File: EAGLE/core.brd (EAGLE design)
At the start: 20.3 x 33 mm, 47 parts, among them Q1 MMDT3904, U1 MIC5219, U3 STM32F10XCXT6, U4 SST25VF040B-Q, X1 USB-MICROB, Y1 8Mhz, Y2 32Khz

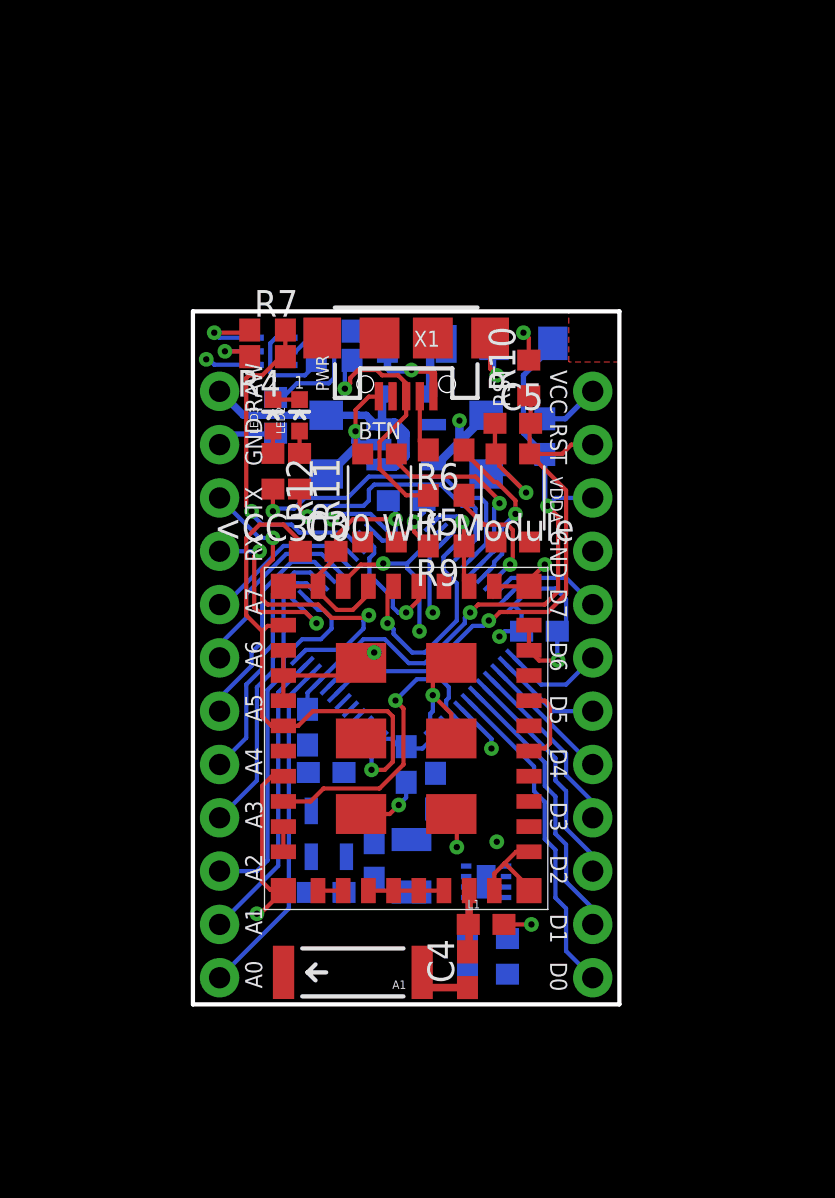
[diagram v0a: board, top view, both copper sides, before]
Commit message: Schematic completed as per latest issues list (Ready for review)
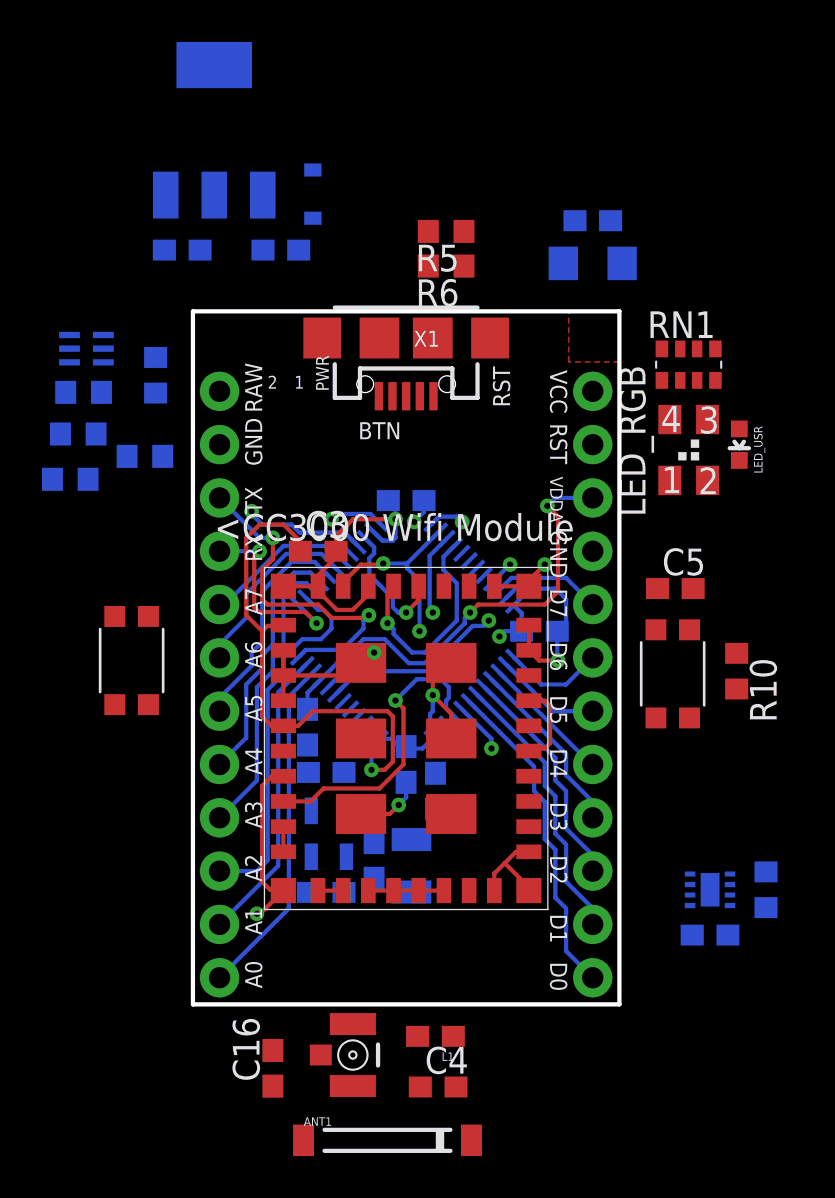
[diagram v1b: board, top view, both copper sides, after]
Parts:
- removed A1: ANTENNA2SMD5, SparkFun-RF:ANTENNA-CHIP5
- removed F1: 500mA, SparkFun:PTC-1206
- removed LED2, LED3: Blue, SparkFun:LED-0603
- removed R11, R12: 1K, rcl:R0603
- removed R9: 10K, rcl:R0603
- removed U1: MIC5219, SparkFun:SOT23-5
- added ANT1: AT8010, Spark:AT8010
- added C16: 10pF, rcl:C0603
- added IC1: MCP1825S-3302E, Spark:SOT223
- added LED_RGB: (no value), Spark:P-LCC-4-3
- added LED_USR: (no value), SparkFun:LED-0603
- added RN1: EXB-38V102JV, resistor-dil:EXB38V
- added X2: IPEX-20279-001E, Spark:IPEX-20279-001E
- C1: value 10uF -> 4.7uF; device SparkFun:EIA3216 -> rcl:C0603
- C2: value 10uF -> 1uF; device SparkFun:EIA3216 -> rcl:C0603
- moved C2 17.2 mm to (-0.51, 35.9), turned to 180 degrees
- moved R10 17.1 mm to (25.9, 15.9), turned to 270 degrees
- moved BTN 14.1 mm to (-2.92, 16.4)
- moved R13 12.7 mm to (27.3, 5.46), turned to 270 degrees
- moved R5 12.6 mm to (12.1, 36.8)
- moved R3 12.0 mm to (-5.21, 29.2)
- moved C6 11.6 mm to (24.6, 3.30), turned to 0 degrees
- moved RESET 11.3 mm to (22.9, 15.7)
- moved R4 11.1 mm to (-5.84, 25.0), flipped to the bottom
- moved C5 11.0 mm to (23.0, 19.8)
- moved R1 10.8 mm to (-2.29, 26.1)
- moved U4 10.7 mm to (24.6, 5.46)
- moved L2 10.5 mm to (19.1, 37.3), turned to 180 degrees
- moved D1 10.5 mm to (5.71, 38.6), turned to 270 degrees
- moved R7 10.3 mm to (-5.46, 27.2), flipped to the bottom
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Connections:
- removed net N$10: LED3.A, R12.1
- removed net N$5: A1.FEED, C4.1
- new net LED3: RN1.7, U3.30
- new net LED4: RN1.8, U3.31
- new net N$14: LED_RGB.4, RN1.1
- new net N$17: LED_RGB.3, RN1.2
- new net N$18: LED_RGB.1, RN1.3
- net +3V3: now also C2.1, IC1.3, LED_RGB.2; no longer C2.A, R9.2, U1.5
- net BTN: now also U3.20; no longer U3.31
- net D7: now also RN1.4
- net GND: now also C1.2, C2.2, IC1.2, IC1.4, LED_USR.C, X2.2@1, X2.2@2; no longer C1.C, C2.C, LED2.C, LED3.C, U1.2
- net LED1: now also LED_USR.A, RN1.5; no longer R11.2, U3.29
- net LED2: now also RN1.6, U3.29; no longer R12.2, U3.30
- net N$2: now also C16.2, X2.1; no longer LED2.A, R11.1
- net N$3: now also ANT1.SIG, C4.1; no longer D1.2, F1.2
- net N$4: now also C16.1
- net RAW: now also C1.1, IC1.1; no longer C1.A, U1.1, U1.3
- net UVCC: now also D1.2; no longer F1.1
- net WIFI_CS: no longer R9.1
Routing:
- net GND: track 94.8 -> 68.1 mm, vias 14 -> 8
- net !RST: track 26.4 -> 8.75 mm
- net LED2: track 15.5 -> 0.00 mm, vias 1 -> 0
- net N$1: track 13.9 -> 0.00 mm, vias 1 -> 0
- net +3V3: track 49.3 -> 35.4 mm, vias 7 -> 4
- net RAW: track 13.6 -> 0.00 mm
- net LED1: track 13.3 -> 0.00 mm, vias 1 -> 0
- net USB_DISC: track 15.8 -> 5.83 mm
- net BTN: track 9.73 -> 0.00 mm, vias 1 -> 0
- net VDDA: track 31.2 -> 22.4 mm
- net N$13: track 8.62 -> 0.00 mm
- net USBM: track 7.73 -> 0.00 mm, vias 1 -> 0
- net UVCC: track 6.46 -> 0.00 mm, vias 1 -> 0
- net USBP: track 6.24 -> 1.25 mm
- net N$16: track 4.96 -> 0.00 mm
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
